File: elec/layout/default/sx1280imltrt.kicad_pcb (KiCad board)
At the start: 2 copper layers, 225.7 x 100.8 mm, 17 parts

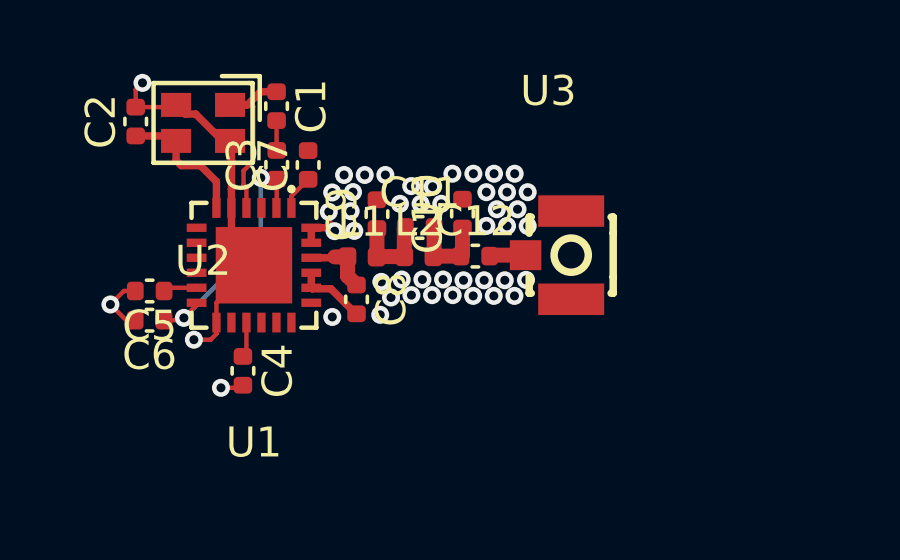
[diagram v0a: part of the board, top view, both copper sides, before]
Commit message: layout
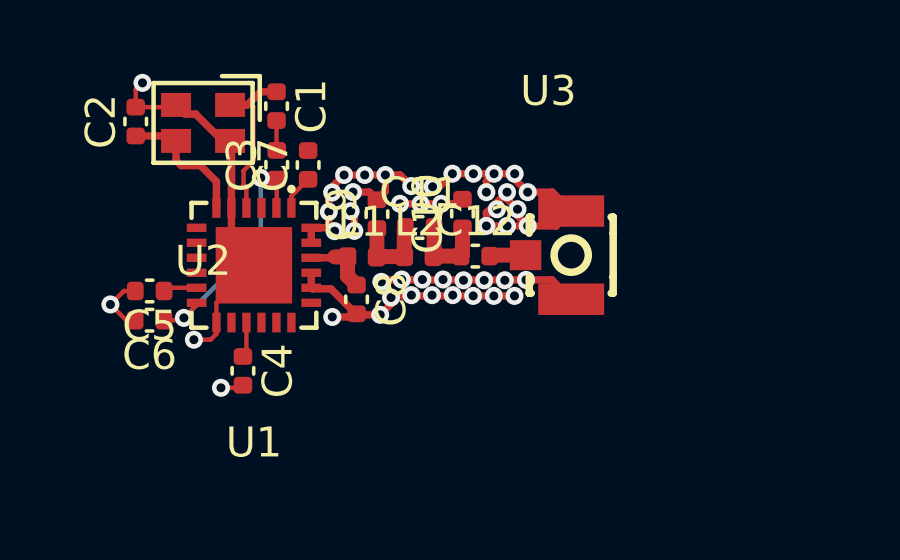
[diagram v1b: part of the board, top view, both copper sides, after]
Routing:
- net gnd: track 21.7 -> 55.4 mm
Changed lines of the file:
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@@
   (segment (start 238.758889 36.556406) (end 239.084059 36.231236) (width 0.15) (layer "F.Cu") (net 4))
   (segment (start 235.163799 33.852629) (end 235.389439 33.626989) (width 0.15) (layer "F.Cu") (net 5))
+  (segment (start 243.674252 40.781355) (end 243.674252 40.99887) (width 0.25) (layer "F.Cu") (net 5))
   (segment (start 241.049736 40.492226) (end 241.669736 40.492226) (width 0.25) (layer "F.Cu") (net 5))
   (segment (start 241.014736 39.957226) (end 241.014736 40.457226) (width 0.25) (layer "F.Cu") (net 5))
   (segment (start 241.657305 40.457226) (end 242.52493 41.324851) (width 0.15) (layer "F.Cu") (net 5))
+  (segment (start 246.853334 37.270742) (end 246.853334 36.910842) (width 0.25) (layer "F.Cu") (net 5))
   (segment (start 238.354736 38.957226) (end 239.104736 39.707226) (width 0.25) (layer "F.Cu") (net 5))
+  (segment (start 249.183409 38.396591) (end 249.68 37.9) (width 0.25) (layer "F.Cu") (net 5))
+  (segment (start 243.485795 36.697662) (end 243.485795 37.242959) (width 0.25) (layer "F.Cu") (net 5))
   (segment (start 237.660448 42.188394) (end 237.103623 42.188394) (width 0.15) (layer "F.Cu") (net 5))
+  (segment (start 242.450556 38.561249) (end 242.450556 38.026133) (width 0.25) (layer "F.Cu") (net 5))
+  (segment (start 245.720314 36.656055) (end 247.796425 36.656055) (width 0.25) (layer "F.Cu") (net 5))
+  (segment (start 248.1737 40.194988) (end 249.034988 40.194988) (width 0.25) (layer "F.Cu") (net 5))
   (segment (start 238.354736 37.797226) (end 238.354736 37.177226) (width 0.25) (layer "F.Cu") (net 5))
   (segment (start 239.859212 34.883761) (end 239.859212 35.872805) (width 0.15) (layer "F.Cu") (net 5))
+  (segment (start 241.716705 41.430604) (end 242.419177 41.430604) (width 0.25) (layer "F.Cu") (net 5))
   (segment (start 237.165453 34.668672) (end 236.815453 34.668672) (width 0.25) (layer "F.Cu") (net 5))
+  (segment (start 247.891039 38.057688) (end 248.229942 38.396591) (width 0.25) (layer "F.Cu") (net 5))
+  (segment (start 247.796425 36.837225) (end 248.229942 37.270742) (width 0.25) (layer "F.Cu") (net 5))
   (segment (start 242.502361 41.324851) (end 242.52493 41.324851) (width 0.25) (layer "F.Cu") (net 5))
   (segment (start 234.845001 41.53826) (end 234.32088 41.014139) (width 0.15) (layer "F.Cu") (net 5))
   (segment (start 238.309059 35.562278) (end 238.059059 35.562278) (width 0.25) (layer "F.Cu") (net 5))
+  (segment (start 243.417291 40.194988) (end 243.351803 40.260476) (width 0.25) (layer "F.Cu") (net 5))
   (segment (start 236.435104 34.436233) (end 236.509059 34.362278) (width 0.15) (layer "F.Cu") (net 5))
   (segment (start 237.854736 41.617226) (end 237.854736 40.957226) (width 0.15) (layer "F.Cu") (net 5))
+  (segment (start 242.406832 37.268148) (end 242.950716 37.268148) (width 0.25) (layer "F.Cu") (net 5))
   (segment (start 238.652708 43.791666) (end 238.738084 43.70629) (width 0.15) (layer "F.Cu") (net 5))
+  (segment (start 245.059449 37.089571) (end 245.286798 37.089571) (width 0.25) (layer "F.Cu") (net 5))
   (segment (start 235.163799 34.436233) (end 236.435104 34.436233) (width 0.15) (layer "F.Cu") (net 5))
+  (segment (start 247.541638 37.270742) (end 247.541638 37.490736) (width 0.25) (layer "F.Cu") (net 5))
   (segment (start 237.854736 41.617226) (end 237.854736 41.994106) (width 0.15) (layer "F.Cu") (net 5))
   (segment (start 238.006063 43.791666) (end 238.652708 43.791666) (width 0.15) (layer "F.Cu") (net 5))
+  (segment (start 247.891039 37.840137) (end 247.891039 38.057688) (width 0.25) (layer "F.Cu") (net 5))
+  (segment (start 245.349031 37.658966) (end 243.972423 37.658966) (width 0.25) (layer "F.Cu") (net 5))
   (segment (start 239.859212 35.872805) (end 239.86474 35.878333) (width 0.15) (layer "F.Cu") (net 5))
+  (segment (start 246.853334 36.910842) (end 247.108121 36.656055) (width 0.25) (layer "F.Cu") (net 5))
+  (segment (start 248.229942 38.396591) (end 249.183409 38.396591) (width 0.25) (layer "F.Cu") (net 5))
+  (segment (start 243.674252 40.99887) (end 243.314251 41.358871) (width 0.25) (layer "F.Cu") (net 5))
   (segment (start 241.669736 40.492226) (end 242.502361 41.324851) (width 0.25) (layer "F.Cu") (net 5))
   (segment (start 241.600711 38.457226) (end 241.600711 37.925447) (width 0.25) (layer "F.Cu") (net 5))
+  (segment (start 247.789244 40.728269) (end 243.727338 40.728269) (width 0.25) (layer "F.Cu") (net 5))
+  (segment (start 245.902997 37.658966) (end 246.056578 37.505385) (width 0.25) (layer "F.Cu") (net 5))
+  (segment (start 246.853334 38.396591) (end 248.229942 38.396591) (width 0.25) (layer "F.Cu") (net 5))
+  (segment (start 245.286798 37.089571) (end 245.720314 36.656055) (width 0.25) (layer "F.Cu") (net 5))
+  (segment (start 248.1737 40.194988) (end 243.417291 40.194988) (width 0.25) (layer "F.Cu") (net 5))
+  (segment (start 242.419177 41.430604) (end 242.52493 41.324851) (width 0.25) (layer "F.Cu") (net 5))
   (segment (start 238.354736 37.797226) (end 238.354736 38.957226) (width 0.25) (layer "F.Cu") (net 5))
+  (segment (start 246.853334 37.959046) (end 247.541638 37.270742) (width 0.25) (layer "F.Cu") (net 5))
   (segment (start 238.059059 35.562278) (end 237.165453 34.668672) (width 0.25) (layer "F.Cu") (net 5))
+  (segment (start 247.541638 37.490736) (end 247.891039 37.840137) (width 0.25) (layer "F.Cu") (net 5))
   (segment (start 238.354736 37.177226) (end 238.358889 37.173073) (width 0.25) (layer "F.Cu") (net 5))
+  (segment (start 243.485795 37.242959) (end 243.205661 37.523093) (width 0.25) (layer "F.Cu") (net 5))
   (segment (start 241.014736 38.457226) (end 241.600711 38.457226) (width 0.25) (layer "F.Cu") (net 5))
   (segment (start 241.014736 40.457226) (end 241.049736 40.492226) (width 0.25) (layer "F.Cu") (net 5))
   (segment (start 237.854736 41.994106) (end 237.660448 42.188394) (width 0.15) (layer "F.Cu") (net 5))
+  (segment (start 243.314251 41.358871) (end 242.55895 41.358871) (width 0.25) (layer "F.Cu") (net 5))
   (segment (start 238.358889 35.612108) (end 238.309059 35.562278) (width 0.25) (layer "F.Cu") (net 5))
   (segment (start 241.014736 38.957226) (end 241.014736 38.457226) (width 0.25) (layer "F.Cu") (net 5))
   (segment (start 235.145247 41.53826) (end 234.845001 41.53826) (width 0.15) (layer "F.Cu") (net 5))
+  (segment (start 248.229942 37.270742) (end 249.050742 37.270742) (width 0.25) (layer "F.Cu") (net 5))
+  (segment (start 241.600711 37.925447) (end 241.600711 37.206138) (width 0.25) (layer "F.Cu") (net 5))
+  (segment (start 245.349031 37.658966) (end 245.902997 37.658966) (width 0.25) (layer "F.Cu") (net 5))
+  (segment (start 242.950716 37.268148) (end 243.205661 37.523093) (width 0.25) (layer "F.Cu") (net 5))
   (segment (start 236.815453 34.668672) (end 236.509059 34.362278) (width 0.25) (layer "F.Cu") (net 5))
+  (segment (start 242.109187 36.697662) (end 243.97654 36.697662) (width 0.25) (layer "F.Cu") (net 5))
+  (segment (start 243.727338 40.728269) (end 243.674252 40.781355) (width 0.25) (layer "F.Cu") (net 5))
   (segment (start 235.163799 34.436233) (end 235.163799 33.852629) (width 0.15) (layer "F.Cu") (net 5))
+  (segment (start 242.55895 41.358871) (end 242.52493 41.324851) (width 0.25) (layer "F.Cu") (net 5))
+  (segment (start 249.034988 40.194988) (end 249.68 40.84) (width 0.25) (layer "F.Cu") (net 5))
+  (segment (start 242.450556 38.026133) (end 242.328512 37.904089) (width 0.25) (layer "F.Cu") (net 5))
   (segment (start 238.358889 37.173073) (end 238.358889 35.612108) (width 0.25) (layer "F.Cu") (net 5))
   (segment (start 235.149689 40.564252) (end 234.770767 40.564252) (width 0.15) (layer "F.Cu") (net 5))
+  (segment (start 247.796425 36.656055) (end 247.796425 36.837225) (width 0.25) (layer "F.Cu") (net 5))
+  (segment (start 241.600711 37.206138) (end 242.109187 36.697662) (width 0.25) (layer "F.Cu") (net 5))
   (segment (start 234.770767 40.564252) (end 234.32088 41.014139) (width 0.15) (layer "F.Cu") (net 5))
   (segment (start 237.854736 40.957226) (end 239.104736 39.707226) (width 0.15) (layer "F.Cu") (net 5))
+  (segment (start 243.97654 36.697662) (end 244.347233 37.068355) (width 0.25) (layer "F.Cu") (net 5))
+  (segment (start 246.853334 38.396591) (end 246.853334 37.959046) (width 0.25) (layer "F.Cu") (net 5))
+  (segment (start 249.050742 37.270742) (end 249.68 37.9) (width 0.25) (layer "F.Cu") (net 5))
   (via (at 243.485795 36.697662) (size 0.6) (drill 0.3) (layers "F.Cu" "B.Cu") (net 5))
   (via (at 247.541638 38.396591) (size 0.6) (drill 0.3) (layers "F.Cu" "B.Cu") (net 5))
